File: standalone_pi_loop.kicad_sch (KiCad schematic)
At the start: 40 parts, among them J1 Conn_01x10_Pin, J10 Vout, J11 PI input select, J2 Conn_01x10_Pin, J3 V-sense, J4 Conn_01x05, J5 pot+, J6 pot-, J7 Setpoint, J8 Alt out, J9 Alt input, U1 AD823, U2 AD620

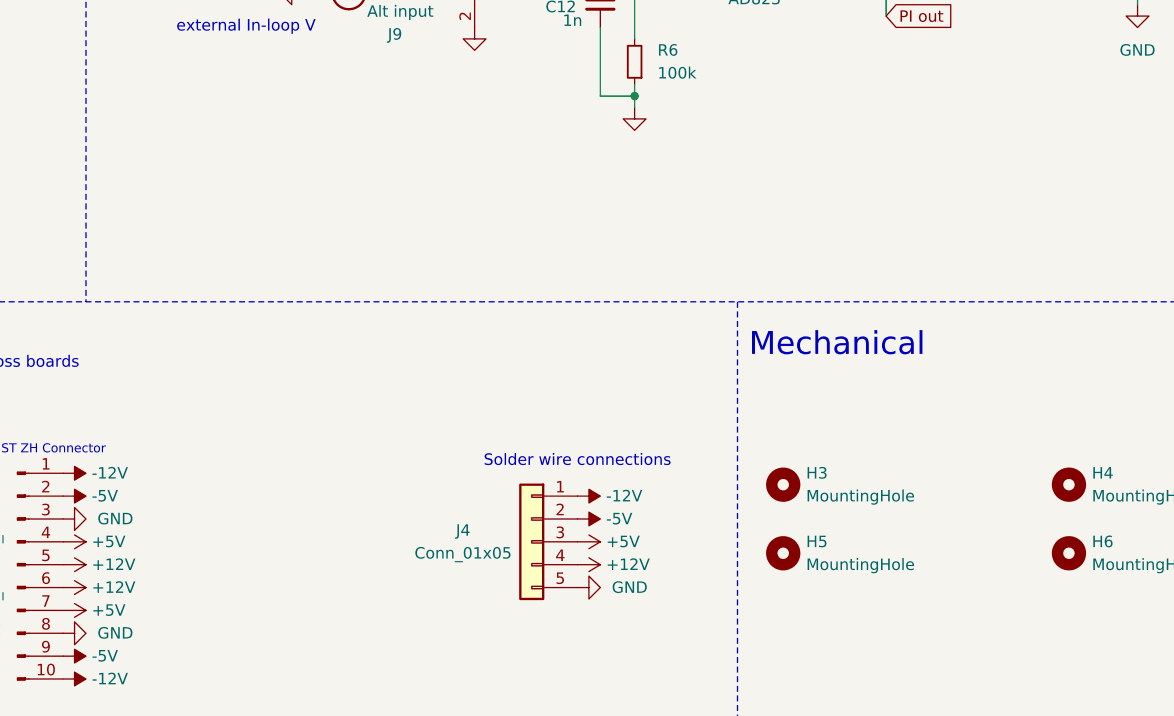
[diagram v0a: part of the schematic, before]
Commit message: Created BOM and pos csv's. Added J4 in pos file
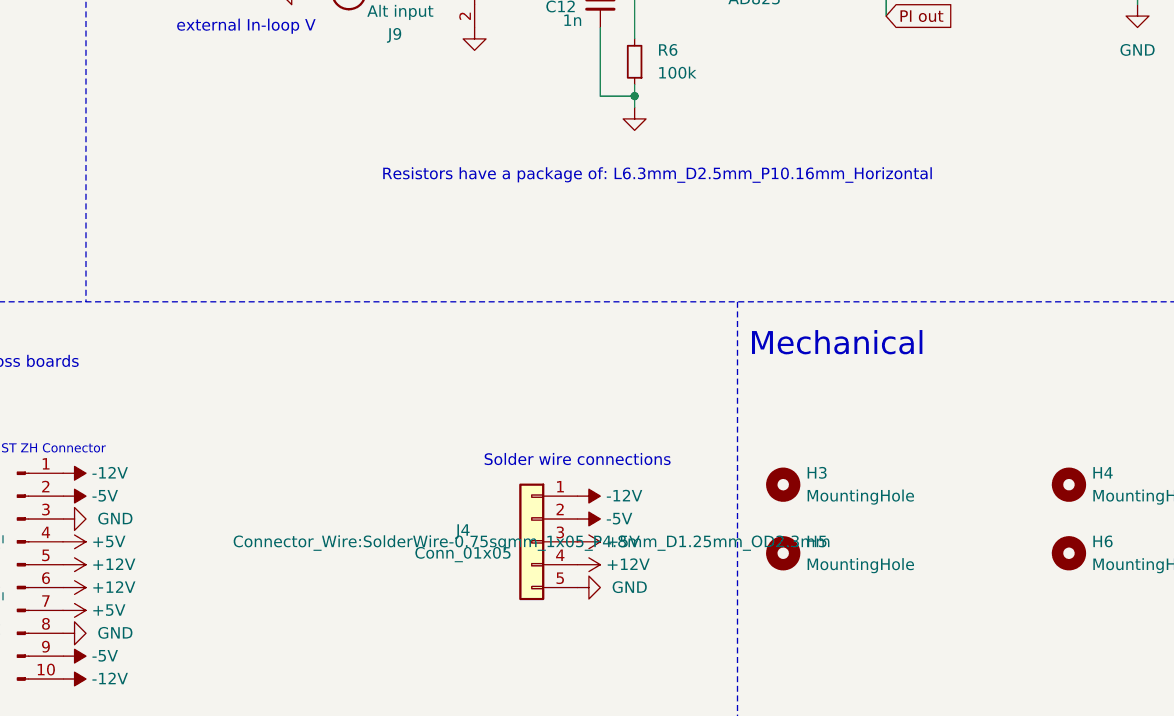
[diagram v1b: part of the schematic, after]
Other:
- note added: "Resistors have a package of: L6.3mm_D2.5mm_P10.16mm_Horizontal"
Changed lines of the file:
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@@
 		)
 	)
+	(text "Resistors have a package of: L6.3mm_D2.5mm_P10.16mm_Horizontal\n"
+		(exclude_from_sim no)
+		(at 123.19 100.33 0)
+		(effects
+			(font
+				(size 1.27 1.27)
+			)
+		)
+	)
 	(text "Current instrumentation amp"
 		(exclude_from_sim no)
@@
 					(size 1.27 1.27)
 				)
-				(hide yes)
 			)
 		)
@@
 			(at 21.59 53.34 0)
 			(effects
+				(font
+					(size 1.27 1.27)
+				)
+				(hide yes)
+			)
+		)
+		(property "LCSC part" ""
+			(at 21.59 53.34 0)
+			(effects
